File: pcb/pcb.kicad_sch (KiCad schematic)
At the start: 7 parts

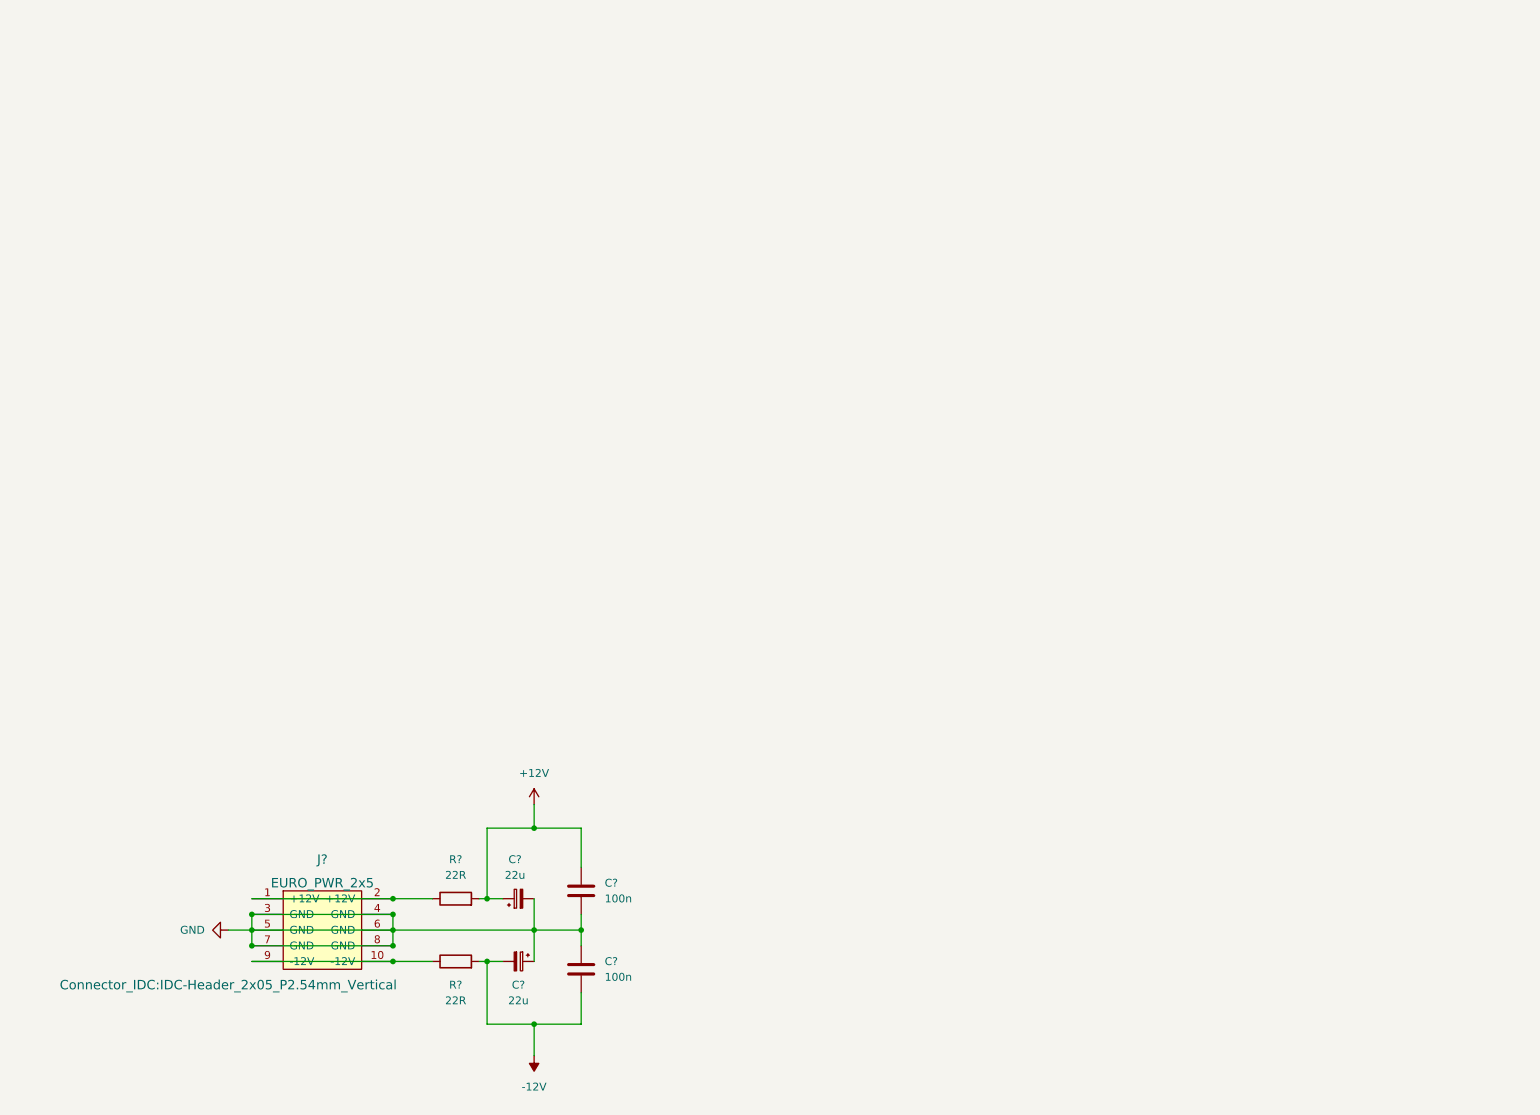
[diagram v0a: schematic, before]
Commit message: WIP
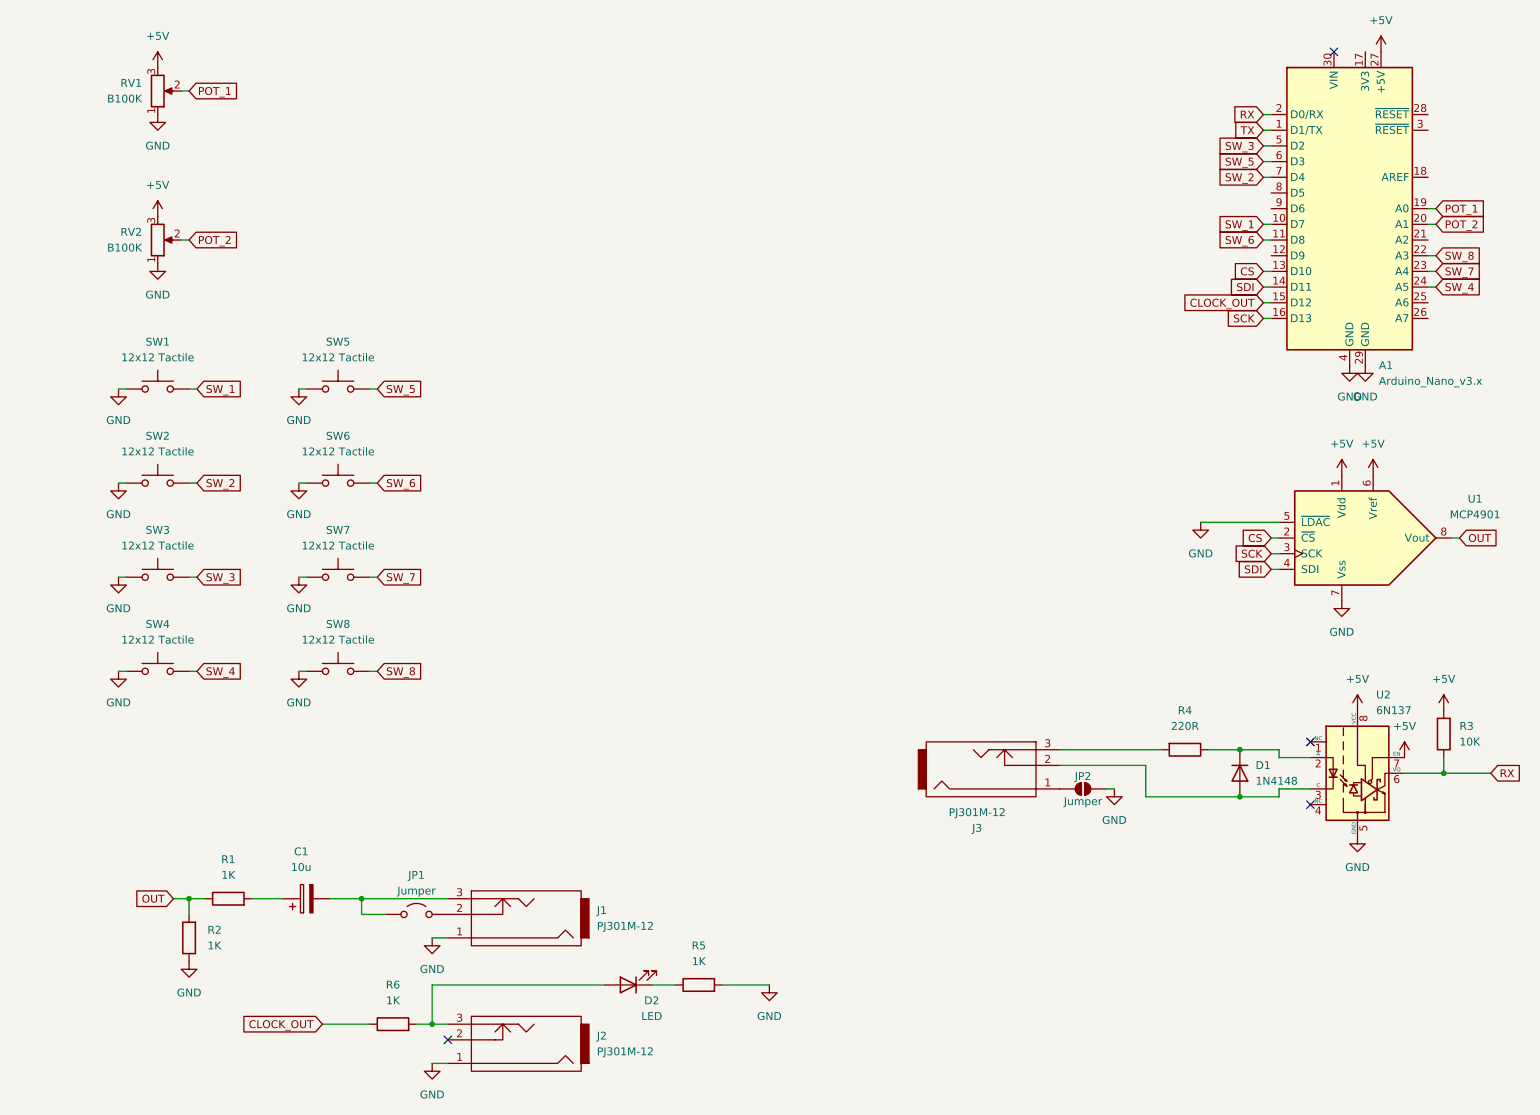
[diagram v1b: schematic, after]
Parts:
- removed C? (x2): 100n, Capacitor_SMD:C_0603_1608Metric, symbol Device:C
- removed C? (x2): 22u, Capacitor_SMD:CP_Elec_4x3.9, symbol Device:C_Polarized_Small
- removed J?: EURO_PWR_2x5, Connector_IDC:IDC-Header_2x05_P2.54mm_Vertical, symbol eurocad:EURO_PWR_2x5
- removed R? (x2): 22R, Resistor_SMD:R_0603_1608Metric, symbol Device:R
- added A1: Arduino_Nano_v3.x, Module:Arduino_Nano, symbol MCU_Module:Arduino_Nano_v3.x
- added C1: 10u, Capacitor_THT:CP_Radial_D5.0mm_P2.50mm, symbol Device:C_Polarized
- added D1: 1N4148, Diode_THT:D_DO-35_SOD27_P7.62mm_Horizontal, symbol Diode:1N4148
- added D2: LED, LED_THT:LED_D5.0mm, symbol Device:LED
- added J1, J2, J3: PJ301M-12, Eurocad:PJ301M-12, symbol eurocad:PJ301M-12
- added JP1: Jumper, TestPoint:TestPoint_2Pads_Pitch2.54mm_Drill0.8mm, symbol Jumper:Jumper_2_Open
- added JP2: Jumper, Jumper:SolderJumper-2_P1.3mm_Open_RoundedPad1.0x1.5mm, symbol Jumper:SolderJumper_2_Open
- added R1, R2, R5, R6: 1K, Resistor_THT:R_Axial_DIN0207_L6.3mm_D2.5mm_P7.62mm_Horizontal, symbol Device:R
- added R3: 10K, Resistor_THT:R_Axial_DIN0207_L6.3mm_D2.5mm_P7.62mm_Horizontal, symbol Device:R
- added R4: 220R, Resistor_THT:R_Axial_DIN0207_L6.3mm_D2.5mm_P7.62mm_Horizontal, symbol Device:R
- added RV1, RV2: B100K, Potentiometer_THT:Potentiometer_Alpha_RD901F-40-00D_Single_Vertical, symbol Device:R_Potentiometer
- added SW1, SW2, SW3, SW4, SW5, SW6, SW7, SW8: 12x12 Tactile, Button_Switch_THT:SW_PUSH-12mm, symbol Switch:SW_Push
- added U1: MCP4901, Package_DIP:DIP-8_W7.62mm, symbol Analog_DAC:MCP4901
- added U2: 6N137, Package_DIP:DIP-8_W7.62mm, symbol Isolator:6N137
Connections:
- net GND: now also A1.29 (GND), A1.4 (GND), J1.1, J2.1, JP2.2 (B), R2.1, R5.2, RV1.1, RV2.1, SW1.1, SW2.1, SW3.1, SW4.1, SW5.1, SW6.1, SW7.1, SW8.1, U1.5 (~{LDAC}), U1.7 (Vss), U2.5 (GND)
- new net: C1.1, R1.2
- new net: J1.2, JP1.2 (B)
- new net: C1.2, J1.3, JP1.1 (A)
- new net: D2.1 (K), R5.1
- new net: D2.2 (A), J2.3, R6.2
- new net: D1.1 (K), R4.1, U2.2 (A)
- new net: D1.2 (A), J3.2, U2.3 (C)
- new net: J3.1, JP2.1 (A)
- new net: J3.3, R4.2
- new net +5V: A1.27 (+5V), R3.2, RV1.3, RV2.3, U1.1 (Vdd), U1.6 (Vref), U2.7 (EN), U2.8 (VCC)
- new net CLOCK_OUT: A1.15 (D12), R6.1
- new net CS: A1.13 (D10), U1.2 (~{CS})
- new net OUT: R1.1, R2.2, U1.8 (Vout)
- new net POT_1: A1.19 (A0), RV1.2
- new net POT_2: A1.20 (A1), RV2.2
- new net RX: A1.2 (D0/RX), R3.1, U2.6 (VO)
- new net SCK: A1.16 (D13), U1.3 (SCK)
- new net SDI: A1.14 (D11), U1.4 (SDI)
- new net SW_1: A1.10 (D7), SW1.2
- new net SW_2: A1.7 (D4), SW2.2
- new net SW_3: A1.5 (D2), SW3.2
- new net SW_4: A1.24 (A5), SW4.2
- new net SW_5: A1.6 (D3), SW5.2
- new net SW_6: A1.11 (D8), SW6.2
- new net SW_7: A1.23 (A4), SW7.2
- new net SW_8: A1.22 (A3), SW8.2
- new net TX: A1.1 (D1/TX)
- no-connect marks 0 -> 4
